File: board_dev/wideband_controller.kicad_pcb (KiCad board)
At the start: 2 copper layers, 35.7 x 34.2 mm, 55 parts, among them J1 Conn_02x05_Odd_Even, J2 Conn_01x06, J3 Conn_01x08, Q1 BTS3028, U1 MCP6004, U2 MCP6004, U4 STM32F042K6Ux, U9 XC6206P332MR

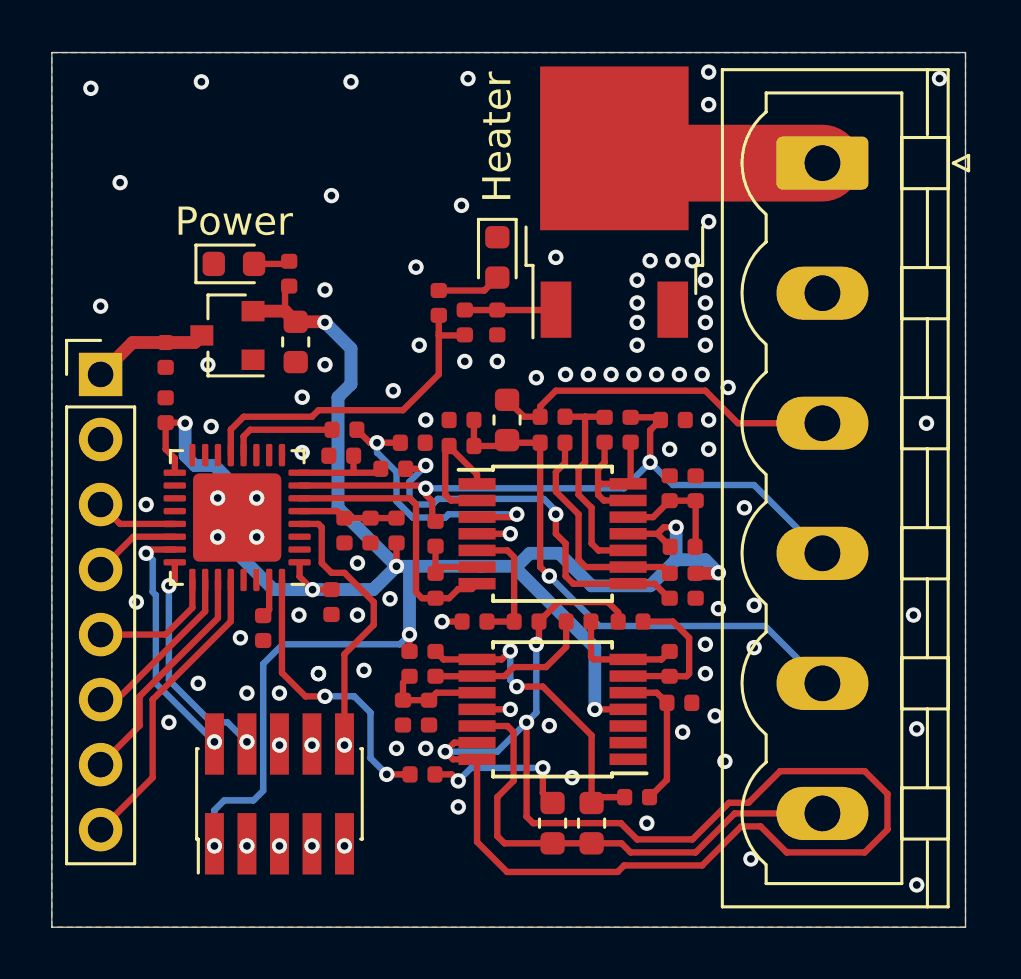
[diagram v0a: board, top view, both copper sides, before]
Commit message: cleanup & tweaks
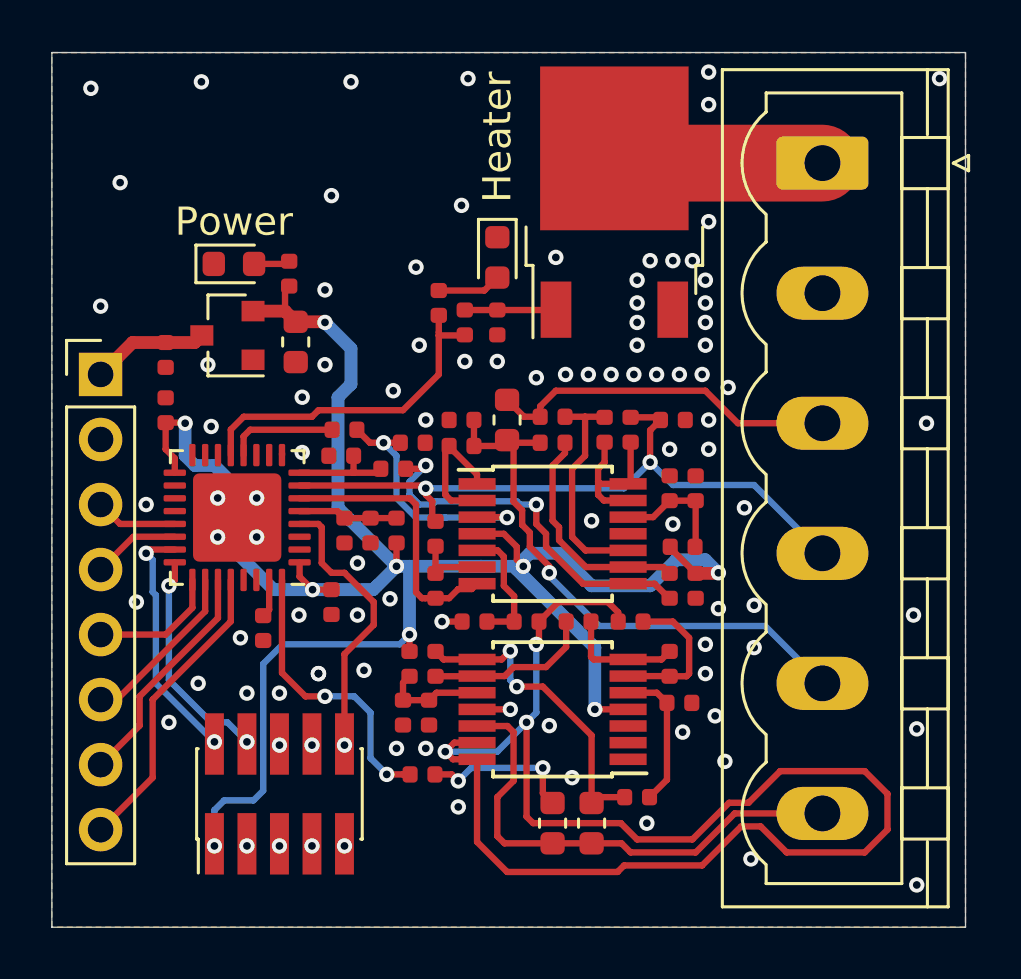
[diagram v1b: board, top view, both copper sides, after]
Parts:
- R1: value 15k -> 10k
- R5, R7: value 30k -> 27k
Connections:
- U1 pad 11: +3V3 -> GND
- U1 pad 4: GND -> +3V3
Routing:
- net GND: track 3.63 -> 2.33 mm, vias 92 -> 93
- net /Ip_dac: track 11.1 -> 10.1 mm
- net /Ip_sense: track 15.6 -> 14.9 mm
- net /LSU_Rtrim: track 21.6 -> 22.2 mm
- net +3V3: track 79.6 -> 80.1 mm
- net Net-(R12-Pad1): track 8.36 -> 8.87 mm
